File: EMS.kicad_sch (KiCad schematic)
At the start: 11 parts, among them J12 Conn_01x02, J13 Conn_01x02, Q4 Q_NMOS_GSD, Q5 Q_PMOS_GSD, Q6 Q_NMOS_GSD

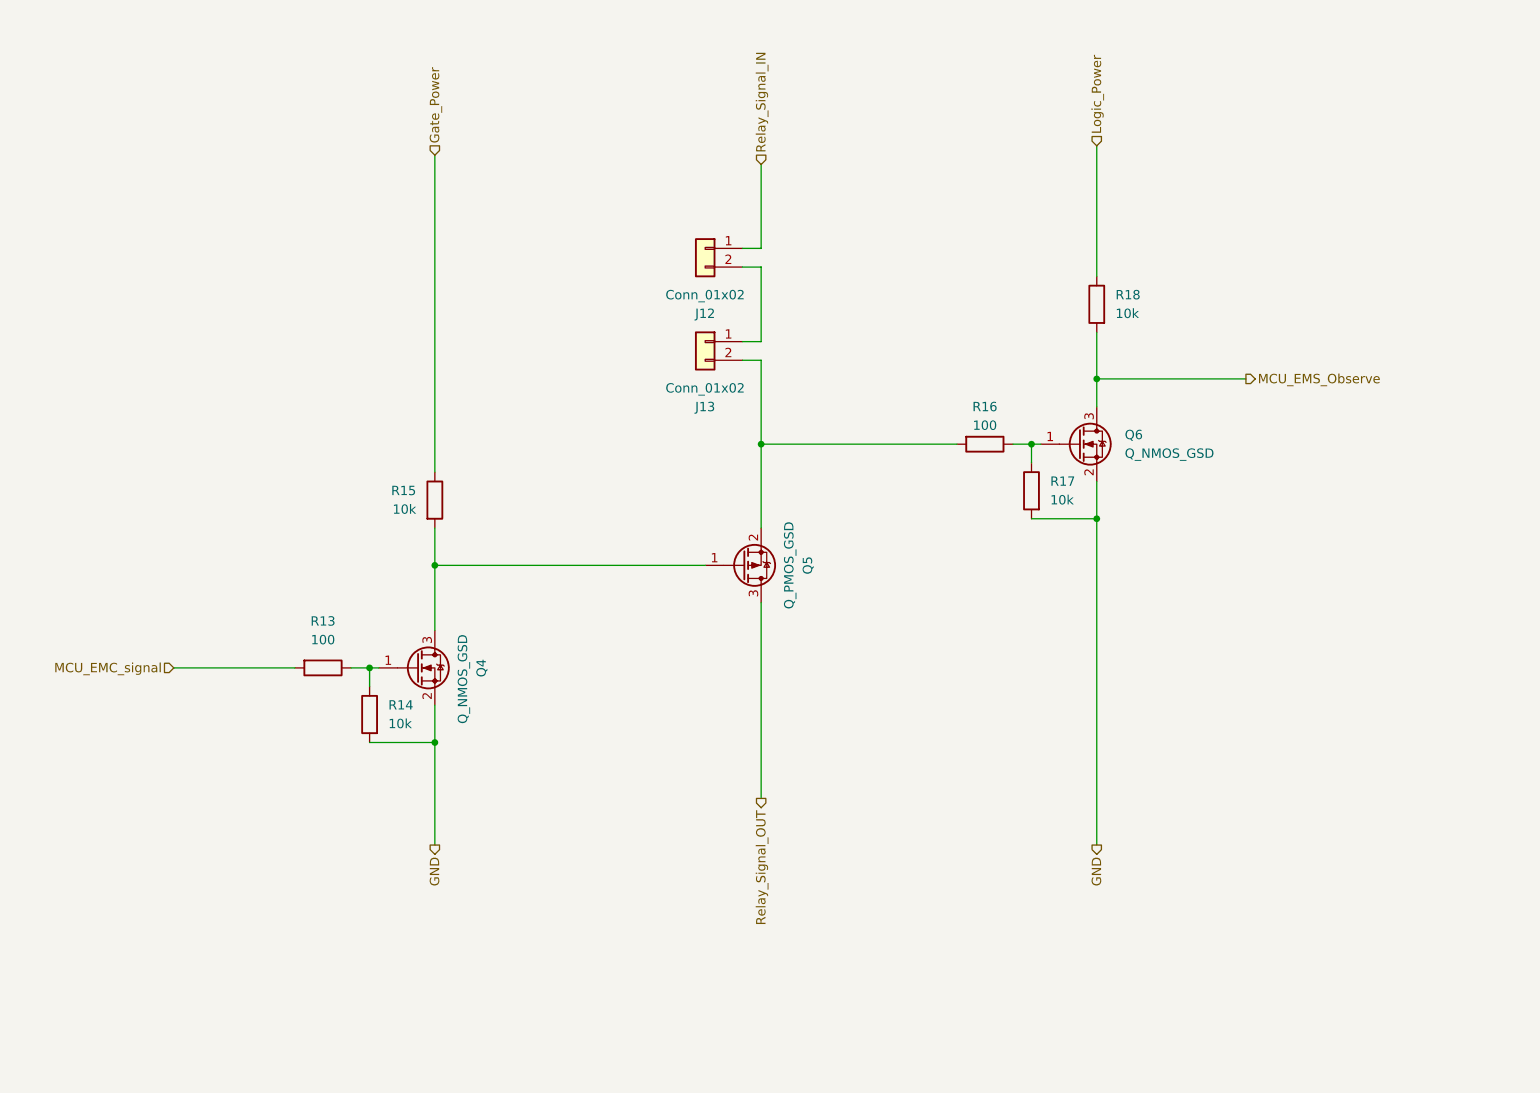
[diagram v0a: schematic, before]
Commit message: precompreate design
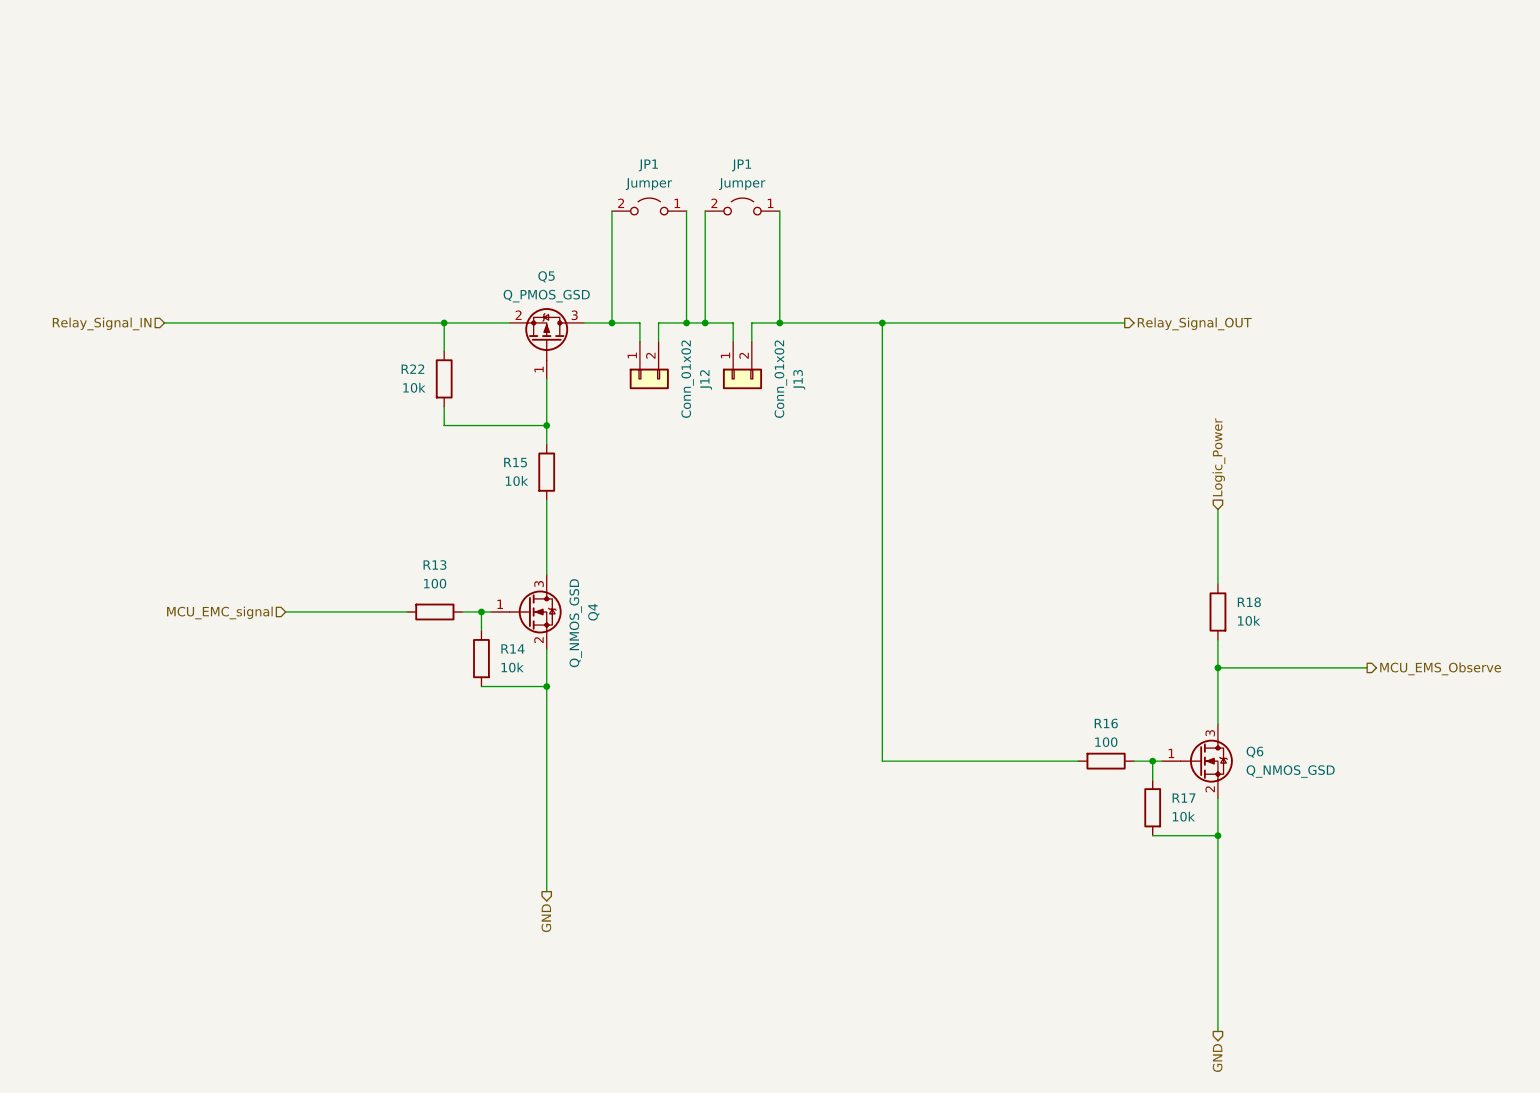
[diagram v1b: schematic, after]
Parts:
- added JP1 (x2): Jumper, Connector_PinHeader_2.54mm:PinHeader_1x02_P2.54mm_Vertical, symbol Jumper:Jumper_2_Open
- added R22: 10k, Resistor_SMD:R_0603_1608Metric_Pad0.98x0.95mm_HandSolder, symbol Device:R
- Q5: footprint Package_TO_SOT_THT:TO-3P-3_Vertical -> Package_TO_SOT_SMD:SOT-23
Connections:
- net Relay_Signal_IN: now also Q5.2 (S), R22.1; no longer J12.1 (Pin_1)
- net Relay_Signal_OUT: now also J13.2 (Pin_2), R16.2, JP1.1 (A); no longer Q5.3 (D)
- net at Q4.3 (D), R15.2: no longer Q5.1 (G)
- net at J12.2 (Pin_2), J13.1 (Pin_1): now also JP1.1 (A), JP1.2 (B)
- net Gate_Power: no longer names the net of R15.1
- net Gate_Power: now also Q5.1 (G), R22.2
- new net: J12.1 (Pin_1), JP1.2 (B), Q5.3 (D)
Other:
- moved on the sheet: Q4, Q6, R13, R14, R15, R16, R17, R18
